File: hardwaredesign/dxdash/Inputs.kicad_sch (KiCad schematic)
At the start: 10 parts, among them J9 Temps

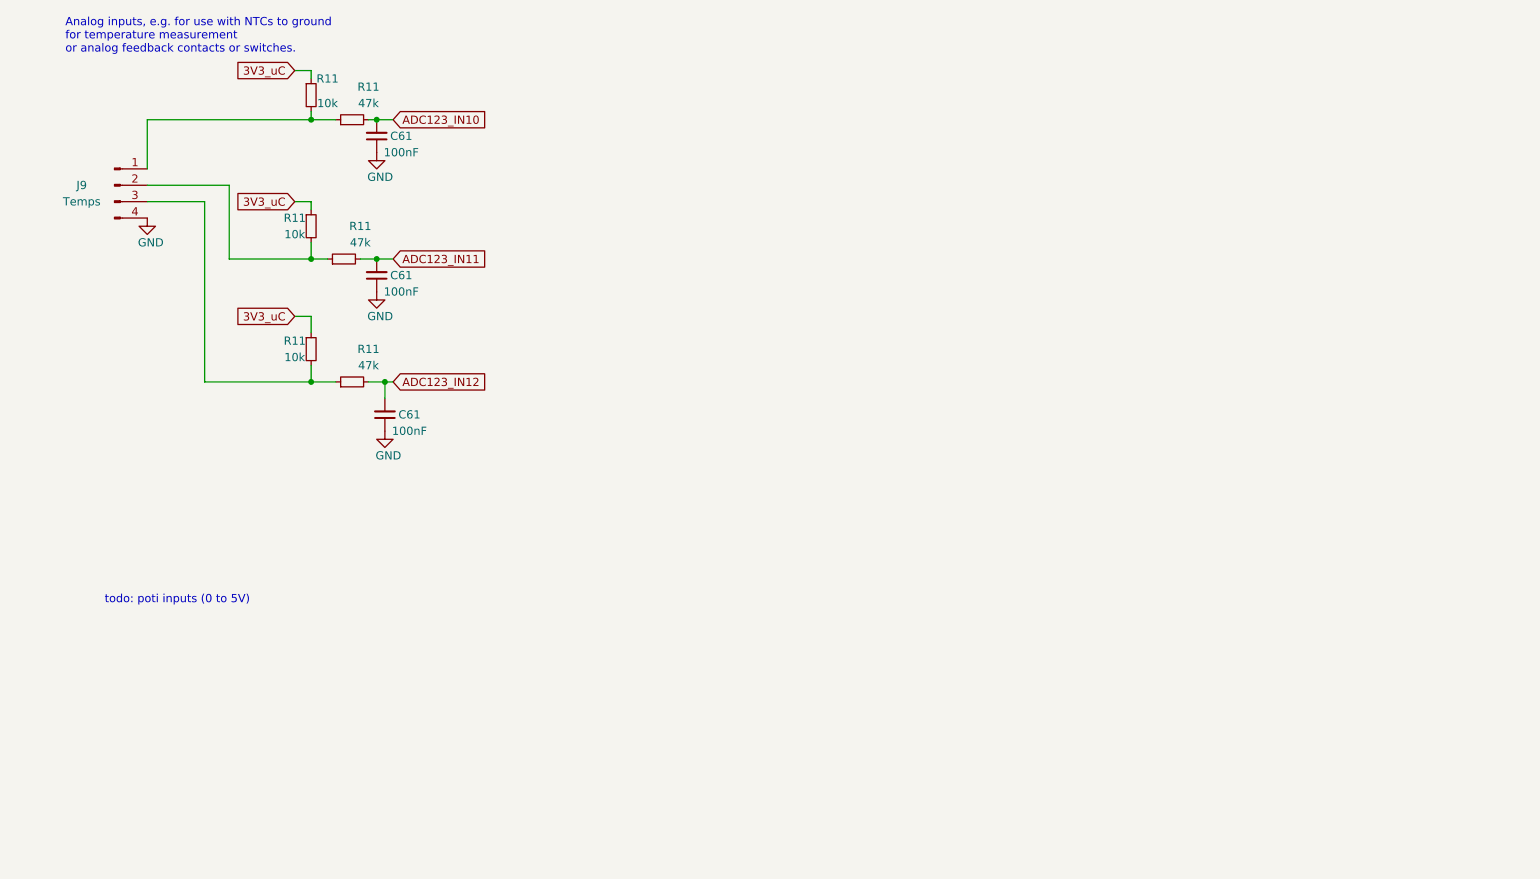
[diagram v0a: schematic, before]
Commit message: controller board added features
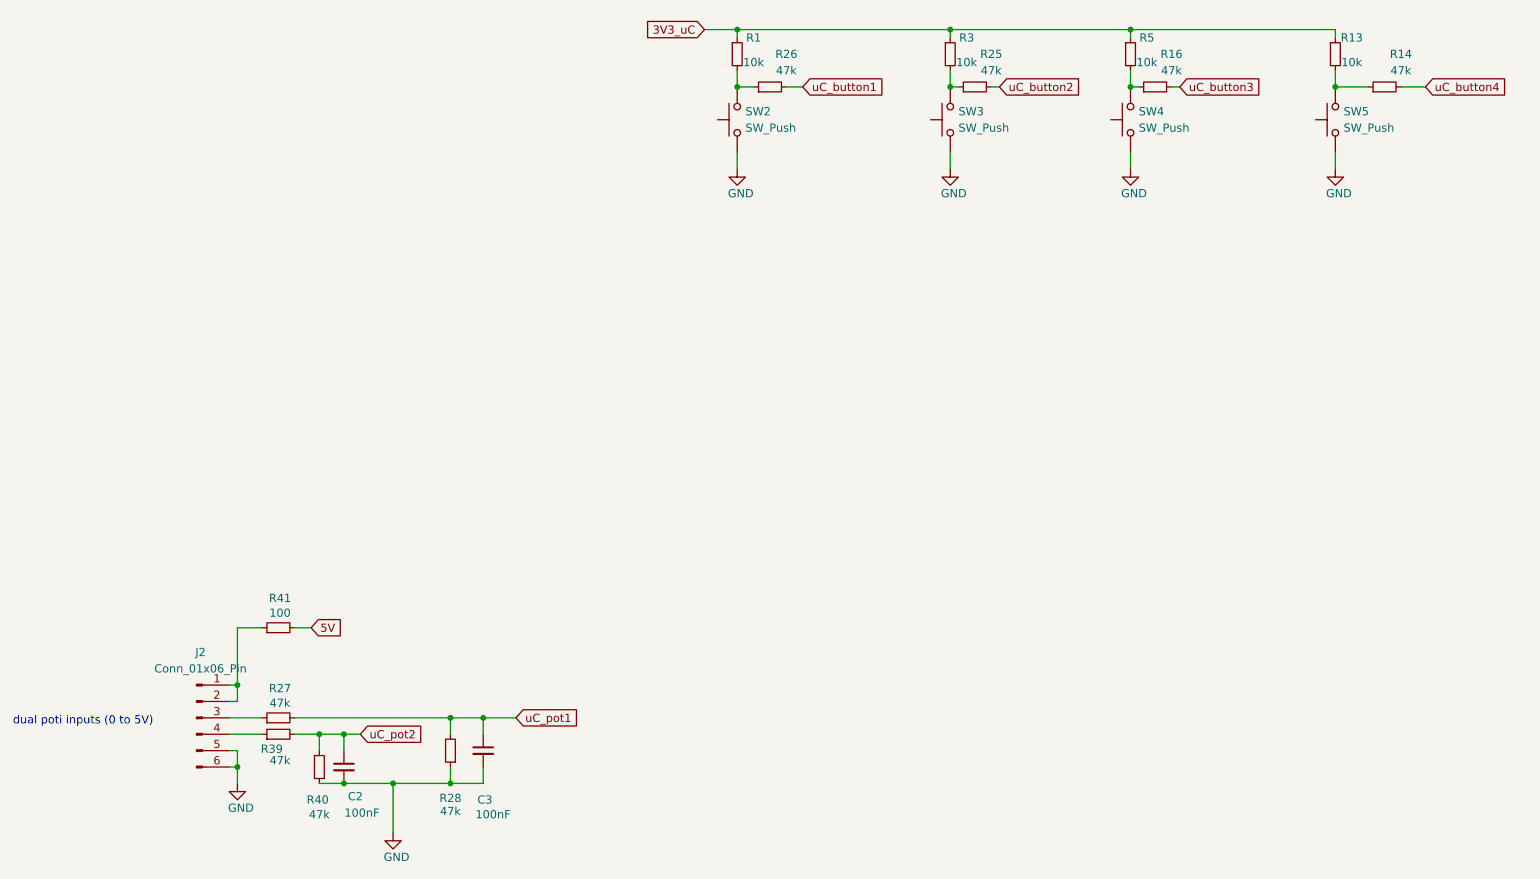
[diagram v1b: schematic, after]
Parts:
- removed C61 (x3): 100nF, Capacitor_SMD:C_1206_3216Metric_Pad1.33x1.80mm_HandSolder, symbol Device:C_Small
- removed J9: Temps, Connector_PinHeader_2.54mm:PinHeader_1x04_P2.54mm_Vertical, symbol Connector:Conn_01x04_Pin
- removed R11 (x3): 47k, Resistor_SMD:R_1206_3216Metric_Pad1.30x1.75mm_HandSolder, symbol Device:R_Small
- removed R11 (x3): 10k, Resistor_SMD:R_1206_3216Metric_Pad1.30x1.75mm_HandSolder, symbol Device:R_Small
- added C2, C3: 100nF, Capacitor_SMD:C_1206_3216Metric_Pad1.33x1.80mm_HandSolder, symbol Device:C_Small
- added J2: Conn_01x06_Pin, Connector_PinHeader_2.54mm:PinHeader_1x06_P2.54mm_Vertical, symbol Connector:Conn_01x06_Pin
- added R1, R13, R3, R5: 10k, Resistor_SMD:R_1206_3216Metric_Pad1.30x1.75mm_HandSolder, symbol Device:R_Small
- added R14, R16, R25, R26, R27, R28, R39, R40: 47k, Resistor_SMD:R_1206_3216Metric_Pad1.30x1.75mm_HandSolder, symbol Device:R_Small
- added R41: 100, Resistor_SMD:R_1206_3216Metric_Pad1.30x1.75mm_HandSolder, symbol Device:R_Small
- added SW2, SW3, SW4, SW5: SW_Push, Button_Switch_THT:SW_PUSH_6mm_H5mm, symbol Switch:SW_Push
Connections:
- net 3V3_uC: now also R1.1, R13.1, R3.1, R5.1
- net GND: now also C2.2, C3.2, J2.5 (Pin_5), J2.6 (Pin_6), R28.1, R40.1, SW2.1, SW3.1, SW4.1, SW5.1
- new net: R1.2, R26.1, SW2.2
- new net: J2.3 (Pin_3), R27.1
- new net: R13.2, R14.1, SW5.2
- new net: R16.1, R5.2, SW4.2
- new net: J2.1 (Pin_1), J2.2 (Pin_2), R41.1
- new net: J2.4 (Pin_4), R39.1
- new net: R25.1, R3.2, SW3.2
- new net 5V: R41.2
- new net uC_button1: R26.2
- new net uC_button2: R25.2
- new net uC_button3: R16.2
- new net uC_button4: R14.2
- new net uC_pot1: C3.1, R27.2, R28.2
- new net uC_pot2: C2.1, R39.2, R40.2
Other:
- note added: "dual poti inputs (0 to 5V)"
- note removed: "Analog inputs, e.g. for use with NTCs to ground for temperature measurement or analog feedback contacts or switches."
- note removed: "todo: poti inputs (0 to 5V)"
